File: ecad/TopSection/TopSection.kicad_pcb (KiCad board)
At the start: 2 copper layers, 101 x 85.5 mm, 171 parts, among them J1 Conn_02x05_Odd_Even, Q1 BSS138, Q10 BSS138, Q2 BSS138, Q3 BSS138, Q4 BSS138, Q5 BSS138, Q6 BSS138, Q7 BSS138, Q8 BSS138, Q9 BSS138, SW1 PEL12T, SW10 Cherry_MX_LED, SW11 PEL12T, SW12 PEL12T, SW13 PEL12T, SW14 PEL12T, SW15 PEL12T, SW16 Cherry_MX_LED, SW17 Cherry_MX_LED, SW18 Cherry_MX_LED, SW19 Cherry_MX_LED, SW2 PEL12T, SW20 Cherry_MX_LED, SW3 PEL12T, SW4 PEL12T, SW5 PEL12T, SW6 Cherry_MX_LED, SW7 Cherry_MX_LED, SW8 Cherry_MX_LED, SW9 Cherry_MX_LED, U1 MCP23S09-xP, U10 TLC5973, U11 TLC5973, U12 TLC5973, U13 TLC5973, U14 TLC5973, U15 TLC5973, U16 TLC5973, U17 TLC5973, U18 TLC5973, U19 TLC5973, U2 MCP23S09-xP, U20 TLC5973, U21 TLC5973, U22 TLC5973, U3 TLC5973, U4 TLC5973, U5 TLC5973, U6 TLC5973, U7 TLC5973, U8 TLC5973, U9 TLC5973

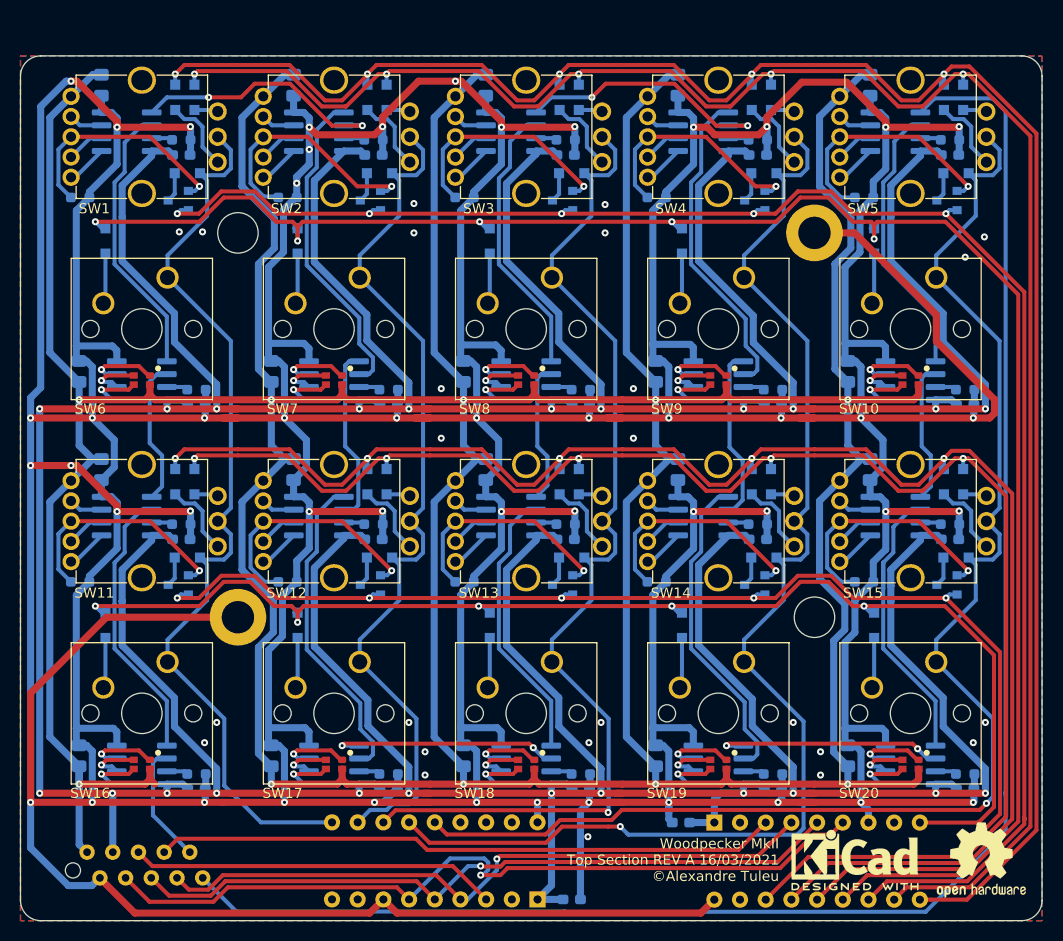
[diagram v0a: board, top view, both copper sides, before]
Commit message: Sets debug board
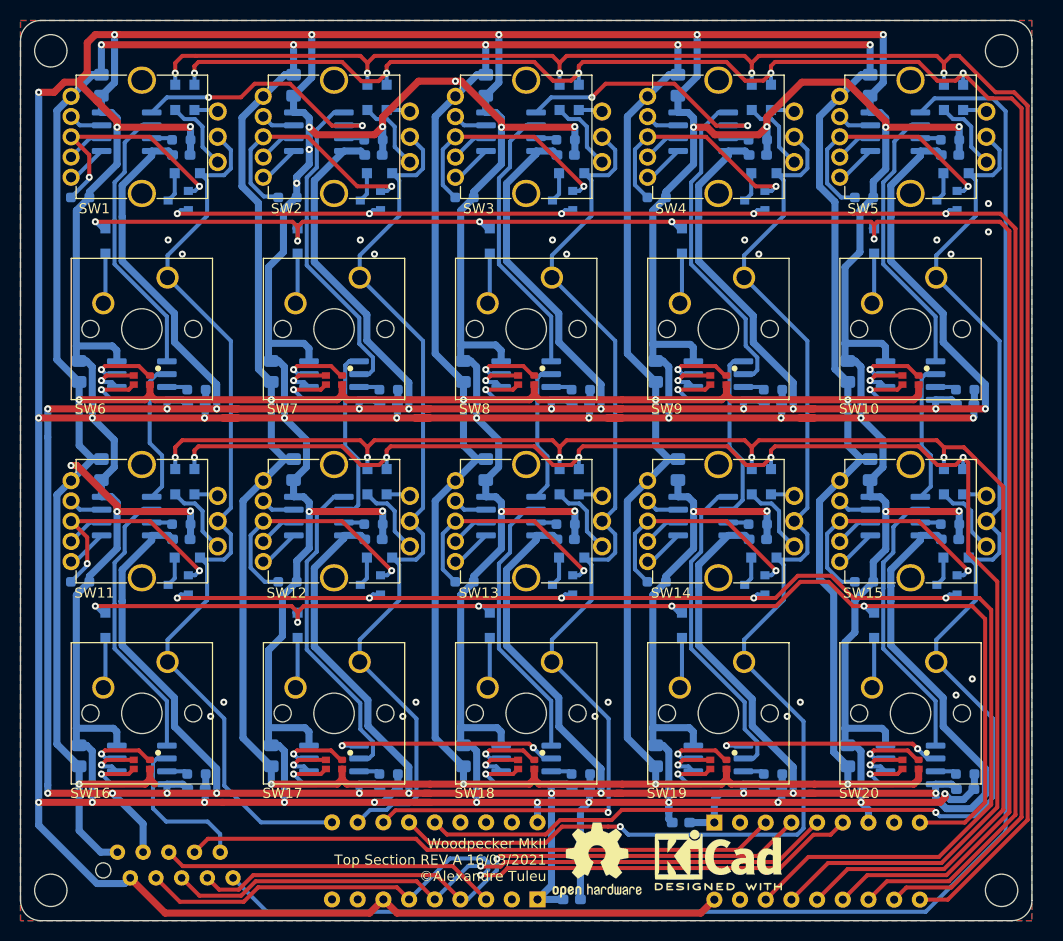
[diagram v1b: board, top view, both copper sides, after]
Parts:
- H1, H2: footprint woodpecker:709620400 -> woodpecker:MountingHole_3.2mm_M3_DIN965
- H3, H4: value MountingHole_Pad -> MountingHole; footprint MountingHole:MountingHole_3.2mm_M3_DIN965_Pad -> woodpecker:MountingHole_3.2mm_M3_DIN965
- moved REF** 38.0 mm to (146.0, 133.5)
- moved H1 32.7 mm to (186.0, 136.5)
- moved H3 32.7 mm to (92.0, 136.5)
- moved H2 25.8 mm to (92.0, 53.5)
- moved H4 25.8 mm to (186.0, 53.5)
- moved REF** 13.5 mm to (158.0, 133.5)
- moved J1 3.00 mm to (104.3, 134.0)
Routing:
- net VLED: track 573.3 -> 658.3 mm, vias 10 -> 15
- net GND: track 1054.8 -> 1097.1 mm, vias 74 -> 75
- net /R3: track 136.1 -> 143.6 mm
- net /QA2: track 156.7 -> 150.6 mm
- net /QB2: track 155.0 -> 149.6 mm
- net /QA1: track 188.5 -> 184.2 mm
- net /QB1: track 186.8 -> 182.8 mm
- net /DI: track 11.9 -> 15.6 mm
- net /MISO: track 79.4 -> 76.4 mm
- net /SCK: track 66.6 -> 63.6 mm
- net /~CS_ROW: track 61.6 -> 58.6 mm
- net /~CS_COL: track 36.3 -> 33.3 mm
- net /MOSI: track 71.1 -> 68.1 mm
- net /DO: track 165.1 -> 162.1 mm
- net /R1: track 168.3 -> 165.7 mm
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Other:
- board size 101 x 85.5 mm -> 100 x 89 mm
